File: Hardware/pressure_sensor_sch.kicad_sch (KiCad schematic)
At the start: 56 parts, among them IC5 ADS131M04IRUKR, J4 1053131104, J5 1053131104, J6 1053131104, J7 1053131104

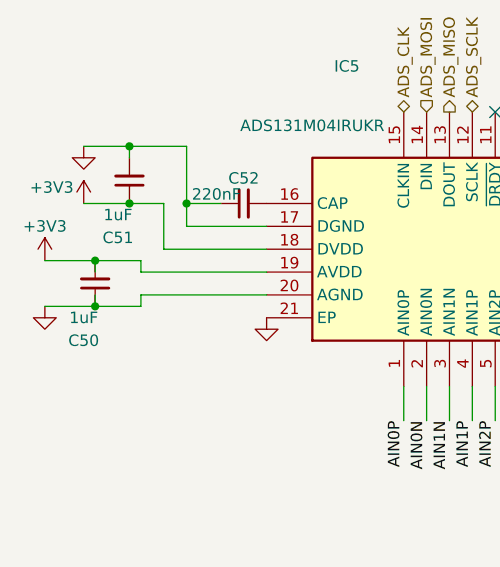
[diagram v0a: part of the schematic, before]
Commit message: update
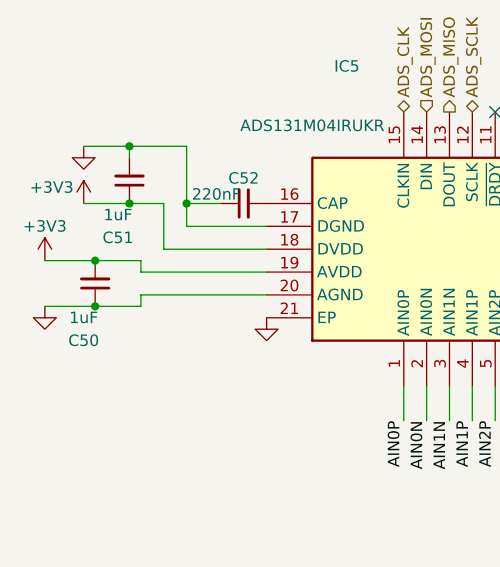
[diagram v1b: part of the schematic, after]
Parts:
- IC5: MPN (none) -> ADS131M04IRUKR
- R35: MPN (none) -> RT0402BRD0775KL
- R37: MPN (none) -> ERA2ARB103X
- R39: MPN (none) -> 0402WGF1402TCE
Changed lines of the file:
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@@
 	(wire
 		(pts
-			(xy 37.592 113.792) (xy 37.592 115.062)
-		)
-		(stroke
-			(width 0)
-			(type default)
-		)
-	)
-	(wire
-		(pts
 			(xy 247.65 62.992) (xy 247.65 68.072)
 		)
@@
 	(wire
 		(pts
-			(xy 37.592 109.982) (xy 37.592 111.252)
-		)
-		(stroke
-			(width 0)
-			(type default)
-		)
-	)
-	(wire
-		(pts
 			(xy 198.628 78.232) (xy 198.628 73.152)
 		)
@@
 			)
 		)
+		(property "MPN" "ADS131M04IRUKR"
+			(at 71.882 123.952 90)
+			(effects
+				(font
+					(size 1.27 1.27)
+				)
+				(hide yes)
+			)
+		)
 		(pin "11"
 		)
@@
 			)
 		)
+		(property "MPN" "RT0402BRD0775KL"
+			(at 170.688 44.45 90)
+			(effects
+				(font
+					(size 1.27 1.27)
+				)
+				(hide yes)
+			)
+		)
 		(pin "1"
 		)
@@
 			)
 		)
+		(property "MPN" "0402WGF1402TCE"
+			(at 170.688 54.864 90)
+			(effects
+				(font
+					(size 1.27 1.27)
+				)
+				(hide yes)
+			)
+		)
 		(pin "1"
 		)
@@
 			(effects
 				(font
+					(size 1.27 1.27)
+				)
+				(hide yes)
+			)
+		)
+		(property "MPN" " ERA2ARB103X"
+			(at 170.688 65.786 90)
+			(effects
+				(font
